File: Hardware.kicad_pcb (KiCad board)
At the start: 2 copper layers, 80 x 40 mm, 0 parts

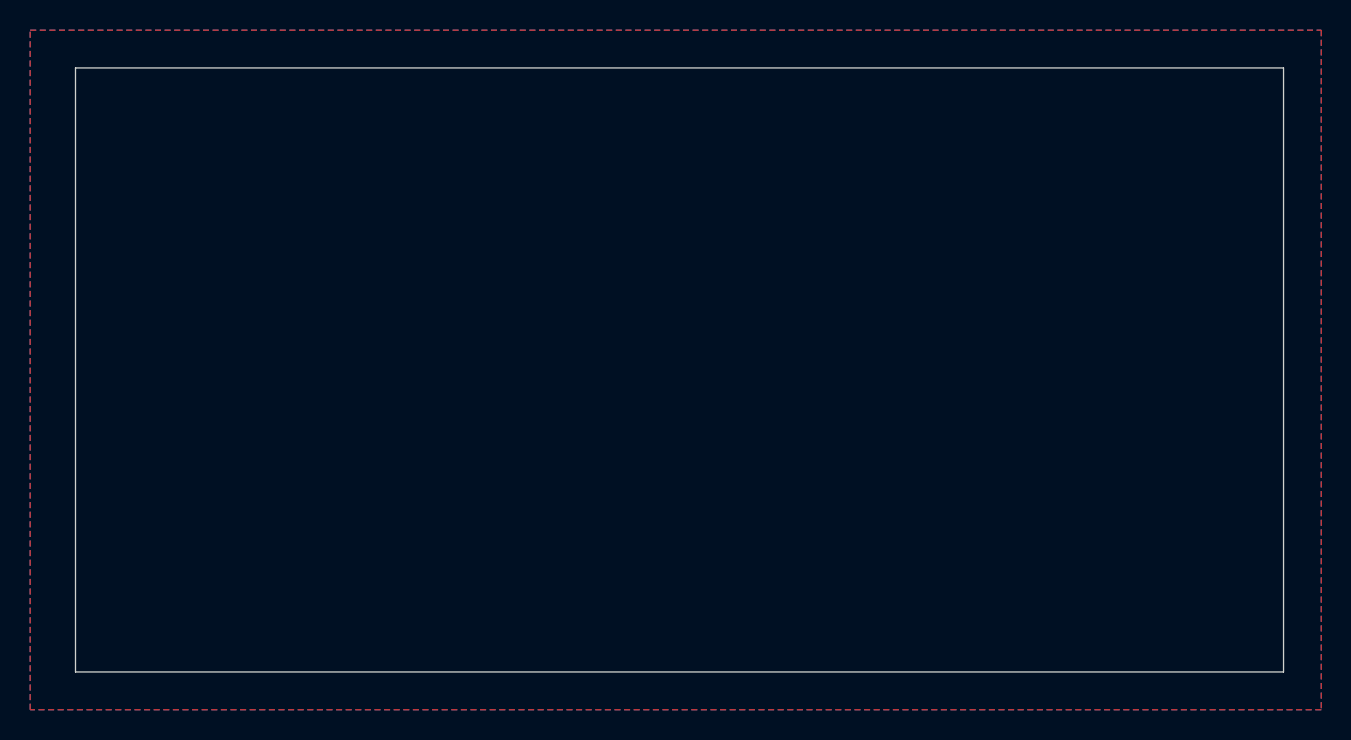
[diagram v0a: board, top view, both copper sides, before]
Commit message: first new layout
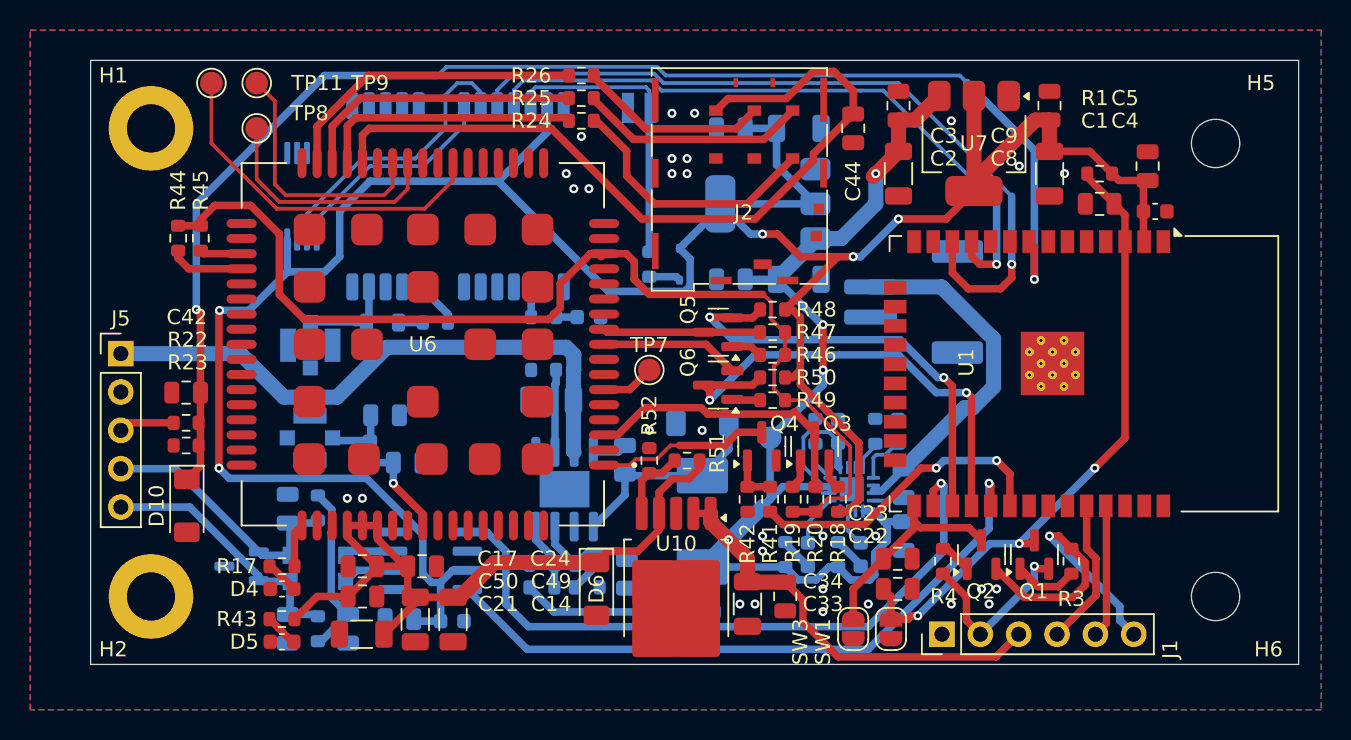
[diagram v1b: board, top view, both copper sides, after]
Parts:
- added BT1: Battery_Cell, Battery:BatteryHolder_Seiko_MS621F, B.Cu at (146.3, 65.1)
- added C1: 100nF, Capacitor_SMD:C_0805_2012Metric, F.Cu at (176.8, 71.5)
- added C10: NC, Capacitor_SMD:C_0805_2012Metric, B.Cu at (131.0, 88.6)
- added C11: NC, Capacitor_SMD:C_0805_2012Metric, B.Cu at (129.5, 85.5)
- added C12: 100nF, Capacitor_SMD:C_0805_2012Metric, B.Cu at (145.4, 88.5)
- added C13: 22uF, Capacitor_SMD:C_0603_1608Metric, B.Cu at (150.5, 98.5)
- added C14: 10uF, Capacitor_SMD:C_1206_3216Metric, F.Cu at (131.5, 99.0)
- added C15: 150pF, Capacitor_SMD:C_0603_1608Metric, B.Cu at (142.9, 95.4)
- added C16: NC, Capacitor_SMD:C_0805_2012Metric, B.Cu at (145.5, 96.0)
- added C17: 100pF, Capacitor_SMD:C_0805_2012Metric, F.Cu at (128.0, 95.5)
- added C18: 100pF, Capacitor_SMD:C_0805_2012Metric, B.Cu at (123.0, 99.6)
- added C19: 100pF, Capacitor_SMD:C_0805_2012Metric, B.Cu at (123.0, 91.7)
- added C2: 10uF, Capacitor_SMD:C_1206_3216Metric, F.Cu at (163.5, 69.5)
- added C20: 4.7uF, Capacitor_SMD:C_0805_2012Metric, B.Cu at (127.0, 99.6)
- added C21: 10uF, Capacitor_SMD:C_1206_3216Metric, F.Cu at (128.0, 100.0)
- added C22: 100nF, Capacitor_SMD:C_0805_2012Metric, F.Cu at (163.4, 97.0)
- added C23: 100nF, Capacitor_SMD:C_0805_2012Metric, F.Cu at (163.4, 95.0)
- added C24: 100pF, Capacitor_SMD:C_0805_2012Metric, F.Cu at (131.9, 95.5)
- added C27: 10uF, Capacitor_SMD:C_1206_3216Metric, B.Cu at (140.5, 84.5)
- added C3: 100pF, Capacitor_SMD:C_0805_2012Metric, F.Cu at (163.5, 65.0)
- added C30: 4.7uF, Capacitor_SMD:C_0805_2012Metric, B.Cu at (163.8, 90.0)
- added C33: 10uF, Capacitor_SMD:C_1206_3216Metric, F.Cu at (153.5, 98.0)
- added C34: 100pF, Capacitor_SMD:C_0805_2012Metric, F.Cu at (156.0, 97.5)
- added C35: 10uF, Capacitor_SMD:C_1206_3216Metric, B.Cu at (156.9, 76.5)
- added C36: 100pF, Capacitor_SMD:C_0805_2012Metric, B.Cu at (152.4, 76.5)
- added C37: 10uF, Capacitor_SMD:C_1206_3216Metric, B.Cu at (156.9, 66.5)
- added C38: 100pF, Capacitor_SMD:C_0805_2012Metric, B.Cu at (152.4, 66.5)
- added C39: 4.7uF, Capacitor_SMD:C_0805_2012Metric, B.Cu at (163.8, 93.5)
- added C4: 22uF, Capacitor_SMD:C_0603_1608Metric, F.Cu at (180.5, 72.0)
- added C42: 100pF, Capacitor_SMD:C_0805_2012Metric, F.Cu at (116.3, 84.0)
- added C44: 100pF, Capacitor_SMD:C_0805_2012Metric, F.Cu at (160.5, 66.5)
- added C46: 1uF, Capacitor_SMD:C_0603_1608Metric, B.Cu at (159.5, 86.6)
- added C49: 10uF, Capacitor_SMD:C_1206_3216Metric, F.Cu at (134.0, 99.0)
- added C5: 100nF, Capacitor_SMD:C_0805_2012Metric, F.Cu at (180.0, 69.0)
- added C50: 100pF, Capacitor_SMD:C_0805_2012Metric, F.Cu at (128.0, 97.5)
- added C6: 22uF, Capacitor_SMD:C_0603_1608Metric, B.Cu at (133.9, 99.1)
- added C7: 100nF, Capacitor_SMD:C_0805_2012Metric, B.Cu at (130.4, 99.0)
- added C8: 10uF, Capacitor_SMD:C_1206_3216Metric, F.Cu at (173.5, 69.5)
- added C9: 100pF, Capacitor_SMD:C_0805_2012Metric, F.Cu at (173.5, 65.0)
- added D1: LED, Capacitor_SMD:C_0603_1608Metric, B.Cu at (143.0, 79.0)
- added D10: BZV55B5V1, Diode_SMD:D_MiniMELF, F.Cu at (116.4, 91.5)
- added D2: 1N4148, Diode_SMD:D_SOD-323, B.Cu at (149.0, 75.5)
- added D3: PESD1CAN, Package_TO_SOT_SMD:SOT-23-3, B.Cu at (120.0, 95.5)
- added D4: LED, Capacitor_SMD:C_0603_1608Metric, F.Cu at (122.7, 97.0)
- added D5: LED, Capacitor_SMD:C_0603_1608Metric, F.Cu at (122.7, 100.5)
- added D6: BZV55B5V1, Diode_SMD:D_MiniMELF, F.Cu at (143.5, 97.0)
- added D7: LED, Capacitor_SMD:C_0603_1608Metric, B.Cu at (161.0, 94.7)
- added D8: LED, Capacitor_SMD:C_0603_1608Metric, B.Cu at (157.5, 94.7)
- added D9: BZV55B5V1, Diode_SMD:D_MiniMELF, B.Cu at (150.5, 86.0)
- added H1: MountingHole_Pad, MountingHole:MountingHole_3.2mm_M3_DIN965_Pad, F.Cu at (114.0, 66.5)
- added H2: MountingHole_Pad, MountingHole:MountingHole_3.2mm_M3_DIN965_Pad, F.Cu at (114.0, 97.5)
- added H5: MountingHole, MountingHole:MountingHole_3.2mm_M3, F.Cu at (184.5, 67.5)
- added H6: MountingHole, MountingHole:MountingHole_3.2mm_M3, F.Cu at (184.5, 97.5)
- added J1: Conn_01x06_Socket, Connector_PinHeader_2.54mm:PinHeader_1x06_P2.54mm_Vertical, F.Cu at (166.4, 100.0)
- added J2: JAE_SIM_Card_SF72S006, Connector_JAE:JAE_SIM_Card_SF72S006, F.Cu at (153.9, 67.8)
- added J3: Conn_Coaxial, Connector_Coaxial:U.FL_Molex_MCRF_73412-0110_Vertical, B.Cu at (124.5, 80.9)
- added J4: Conn_Coaxial, Connector_Coaxial:U.FL_Molex_MCRF_73412-0110_Vertical, B.Cu at (124.5, 87.0)
- added J5: Conn_01x05_Socket, Connector_PinHeader_2.54mm:PinHeader_1x05_P2.54mm_Vertical, F.Cu at (112.0, 81.4)
- added J9: Battery, Connector_JST:JST_PH_S2B-PH-SM4-TB_1x02-1MP_P2.00mm_Horizontal, B.Cu at (164.5, 78.0)
- added L1: 27uH, Inductor_SMD:L_0805_2012Metric, B.Cu at (129.3, 79.4)
- added L2: 15uH, Inductor_SMD:L_Abracon_ASPI-0630LR, B.Cu at (150.5, 92.5)
- added L4: EPCO B82787C0513, EPCO_B82787C0513:EPCO B82787C0513, B.Cu at (125.0, 95.6)
- added Q1: BC849, Package_TO_SOT_SMD:SOT-23, F.Cu at (172.5, 94.7)
- added Q2: BC849, Package_TO_SOT_SMD:SOT-23, F.Cu at (169.0, 94.7)
- added Q3: MMBT3904, Package_TO_SOT_SMD:SOT-23, F.Cu at (157.9, 87.6)
- added Q4: BC849, Package_TO_SOT_SMD:SOT-23, F.Cu at (154.4, 87.6)
- added Q5: MMBT3904, Package_TO_SOT_SMD:SOT-23, F.Cu at (151.6, 80.0)
- added Q6: MMBT3904, Package_TO_SOT_SMD:SOT-23, F.Cu at (151.6, 83.5)
- added R1: 10K, Resistor_SMD:R_0603_1608Metric, F.Cu at (176.8, 69.5)
- added R10: 60R, Resistor_SMD:R_0603_1608Metric, B.Cu at (125.0, 91.6)
- added R11: 60R, Resistor_SMD:R_0603_1608Metric, B.Cu at (125.0, 99.6)
- added R12: 120R, Resistor_SMD:R_0603_1608Metric, B.Cu at (147.0, 75.5)
- added R13: R33, Resistor_SMD:R_0603_1608Metric, B.Cu at (128.5, 88.0)
- added R14: 10K, Resistor_SMD:R_0603_1608Metric, B.Cu at (163.5, 86.6)
- added R15: 40K2, Resistor_SMD:R_0603_1608Metric, B.Cu at (139.9, 95.4)
- added R16: 210K, Resistor_SMD:R_0603_1608Metric, B.Cu at (139.9, 96.9)
- added R17: 51R, Resistor_SMD:R_0603_1608Metric, F.Cu at (122.7, 95.5)
- added R18: 100K, Resistor_SMD:R_0603_1608Metric, F.Cu at (159.5, 91.1)
- added R19: 4K7, Resistor_SMD:R_0603_1608Metric, F.Cu at (156.5, 91.1)
- added R2: 1K, Resistor_SMD:R_0603_1608Metric, B.Cu at (159.5, 94.7)
- added R20: 4K7, Resistor_SMD:R_0603_1608Metric, F.Cu at (158.0, 91.1)
- added R21: 100K, Resistor_SMD:R_0603_1608Metric, B.Cu at (142.9, 96.9)
- added R22: 10K, Resistor_SMD:R_0603_1608Metric, F.Cu at (116.3, 86.0)
- added R23: 3K9, Resistor_SMD:R_0603_1608Metric, F.Cu at (116.3, 87.5)
- added R24: 22R, Resistor_SMD:R_0603_1608Metric, F.Cu at (142.5, 66.0)
- added R25: 22R, Resistor_SMD:R_0603_1608Metric, F.Cu at (142.5, 64.5)
- added R26: 22R, Resistor_SMD:R_0603_1608Metric, F.Cu at (142.5, 63.0)
- added R27: 100K, Resistor_SMD:R_0603_1608Metric, B.Cu at (140.0, 82.5)
- added R3: 10K, Resistor_SMD:R_0603_1608Metric, F.Cu at (174.9, 95.2)
- added R4: 10K, Resistor_SMD:R_0603_1608Metric, F.Cu at (166.4, 95.2)
- added R41: 4K7, Resistor_SMD:R_0603_1608Metric, F.Cu at (155.0, 91.1)
- added R42: 47K, Resistor_SMD:R_0603_1608Metric, F.Cu at (153.5, 91.1)
- added R43: 51R, Resistor_SMD:R_0603_1608Metric, F.Cu at (122.7, 99.0)
- added R44: 1K, Resistor_SMD:R_0603_1608Metric, F.Cu at (115.8, 73.8)
- added R45: 1K, Resistor_SMD:R_0603_1608Metric, F.Cu at (117.3, 73.8)
- added R46: 4K7, Resistor_SMD:R_0603_1608Metric, F.Cu at (155.2, 81.5)
- added R47: 4K7, Resistor_SMD:R_0603_1608Metric, F.Cu at (155.2, 80.0)
- added R48: 100K, Resistor_SMD:R_0603_1608Metric, F.Cu at (155.2, 78.5)
- added R49: 4K7, Resistor_SMD:R_0603_1608Metric, F.Cu at (155.2, 84.5)
- added R5: 1K, Resistor_SMD:R_0603_1608Metric, B.Cu at (156.0, 94.7)
- added R50: 4K7, Resistor_SMD:R_0603_1608Metric, F.Cu at (155.2, 83.0)
- added R51: 22K, Resistor_SMD:R_0603_1608Metric, F.Cu at (149.5, 88.5)
- added R52: 10K, Resistor_SMD:R_0603_1608Metric, F.Cu at (147.0, 88.5)
- added R6: 1k18, Resistor_SMD:R_0603_1608Metric, B.Cu at (158.0, 86.6)
- added R7: 1k13, Resistor_SMD:R_0603_1608Metric, B.Cu at (162.0, 86.6)
- added R8: 22R, Resistor_SMD:R_0603_1608Metric, B.Cu at (132.8, 79.4)
- added R9: 1K, Resistor_SMD:R_0603_1608Metric, B.Cu at (140.0, 79.0)
- added SW1: SW_Push, Jumper:SolderJumper-2_P1.3mm_Open_RoundedPad1.0x1.5mm, F.Cu at (163.0, 99.7)
- added SW3: SW_Push, Jumper:SolderJumper-2_P1.3mm_Open_RoundedPad1.0x1.5mm, F.Cu at (160.5, 99.7)
- added TP11: TestPoint, TestPoint:TestPoint_Pad_D1.5mm, F.Cu at (118.0, 63.5)
- added TP2: TestPoint, TestPoint:TestPoint_Pad_D1.5mm, B.Cu at (155.0, 87.0)
- added TP7: TestPoint, TestPoint:TestPoint_Pad_D1.5mm, F.Cu at (147.0, 82.5)
- added TP8: TestPoint, TestPoint:TestPoint_Pad_D1.5mm, F.Cu at (121.0, 66.5)
- added TP9: TestPoint, TestPoint:TestPoint_Pad_D1.5mm, F.Cu at (121.0, 63.5)
- added U1: ESP32-WROOM-32, RF_Module:ESP32-WROOM-32, F.Cu at (172.8, 82.8)
- added U10: MIC29302AWD, Package_TO_SOT_SMD:TO-252-5_TabPin3, F.Cu at (148.8, 97.0)
- added U11: AMS1117-3.3, Package_TO_SOT_SMD:SOT-223-3_TabPin2, B.Cu at (154.8, 71.5)
- added U2: NEO-M8M, RF_GPS:ublox_NEO, B.Cu at (134.3, 71.0)
- added U3: SN65HVD231, Package_SO:SOIC-8_3.9x4.9mm_P1.27mm, B.Cu at (132.5, 95.1)
- added U4: BQ24075RGT, Package_DFN_QFN:VQFN-16-1EP_3x3mm_P0.5mm_EP1.6x1.6mm, B.Cu at (160.4, 90.4)
- added U5: AT24CS01-XHM, Package_SO:TSSOP-8_4.4x3mm_P0.65mm, B.Cu at (124.0, 71.0)
- added U6: A7670E, A7670E:A7670E, F.Cu at (132.0, 80.8)
- added U7: AMS1117-3.3, Package_TO_SOT_SMD:SOT-223-3_TabPin2, F.Cu at (168.5, 67.5)
- added U8: MP1584EN, SOIC127P600X170-9N:SOIC127P600X170-9N, B.Cu at (141.4, 90.4)
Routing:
- net +3V3: track 0.00 -> 175.5 mm, vias 0 -> 5
- net +5V: track 0.00 -> 121.6 mm, vias 0 -> 4
- net /ACC_Readout: track 0.00 -> 91.5 mm, vias 0 -> 2
- net /LTE_Module/1V8: track 0.00 -> 72.1 mm
- net /LTE_Module/SIM_VCC: track 0.00 -> 52.4 mm
- net GPS_TX: track 0.00 -> 50.9 mm, vias 0 -> 1
- net /LTE_Module/VBAT: track 0.00 -> 47.3 mm
- net CAN_TX: track 0.00 -> 44.6 mm, vias 0 -> 1
- net CAN_RX: track 0.00 -> 44.0 mm, vias 0 -> 1
- net GPS_RX: track 0.00 -> 43.4 mm, vias 0 -> 1
- net /EN: track 0.00 -> 42.1 mm, vias 0 -> 3
- net PW+: track 0.00 -> 39.2 mm
- net LTE_TX: track 0.00 -> 32.0 mm, vias 0 -> 2
- net LTE_RX: track 0.00 -> 29.4 mm, vias 0 -> 2
- net +BATT: track 0.00 -> 24.1 mm
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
